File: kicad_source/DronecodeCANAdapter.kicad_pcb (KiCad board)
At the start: 2 copper layers, 65 x 30 mm, 31 parts, among them CN1 RASPI-IO, CN2 691322310004, CN3 GH_SM04B-GHS-TB, CN4 GH_SM04B-GHS-TB, SW1 JS202011JCQN, U1 MCP2518FD, U2 TCAN332GDR, Y1 RH100-20.000-20-3030-TR

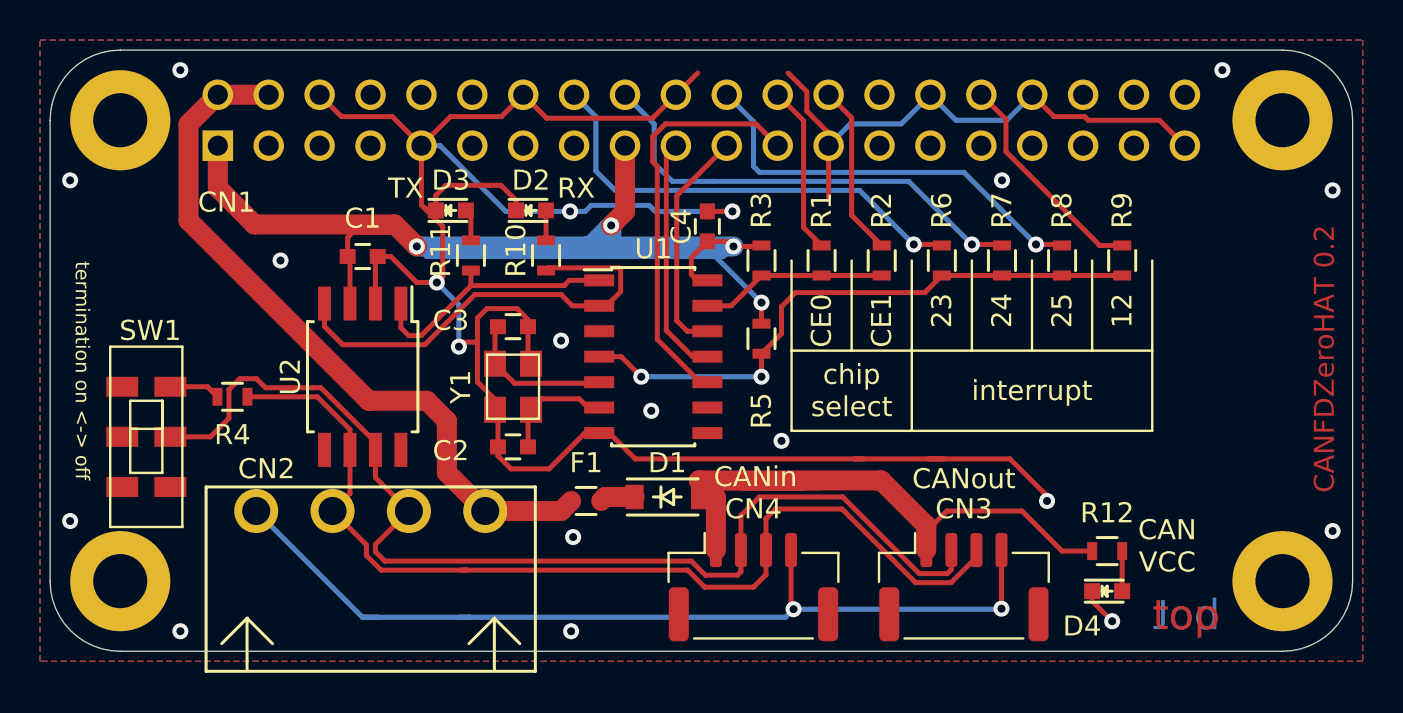
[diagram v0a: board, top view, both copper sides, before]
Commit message: updated schematic and layout
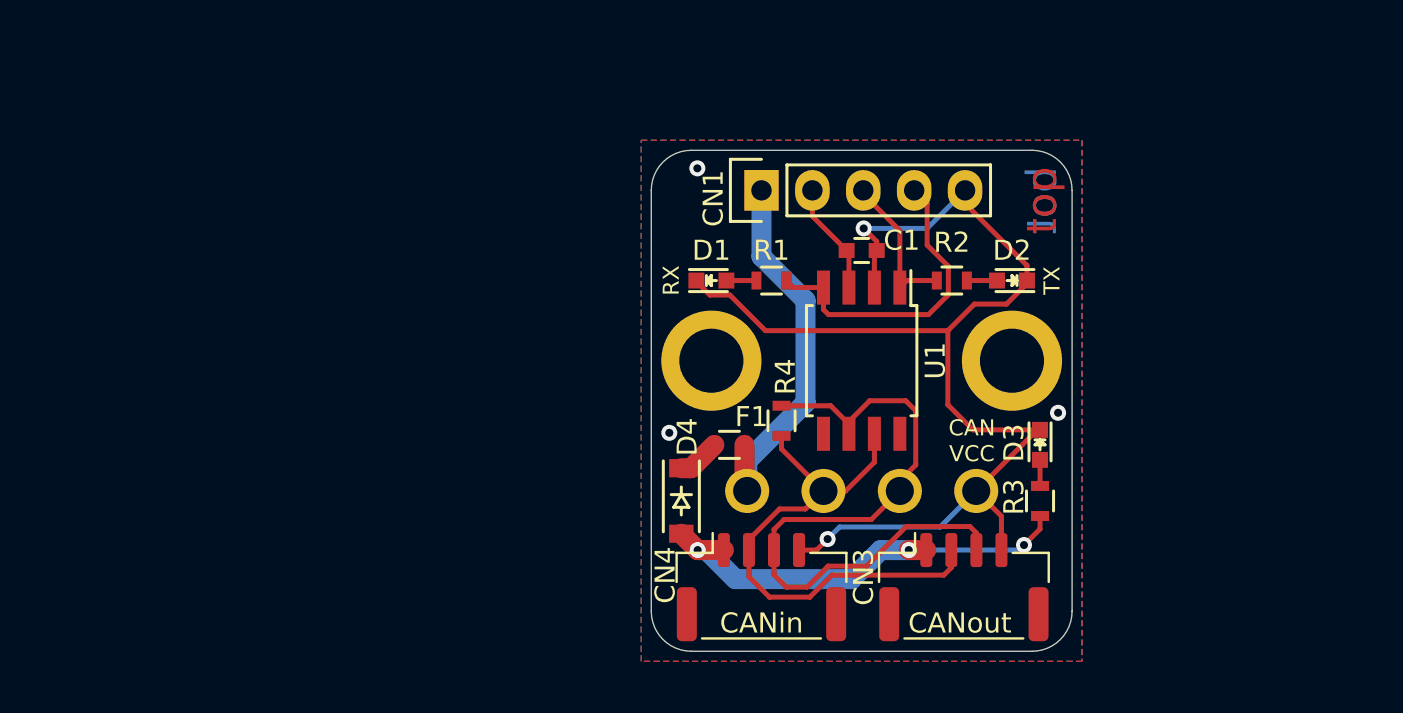
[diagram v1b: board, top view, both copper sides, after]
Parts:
- removed C2, C3: 22pF, capacitors:C_0603
- removed C4: 100nF, capacitors:C_0603
- removed the D3 at (127.5, 94.5)
- removed L2: Label, labels:generationmake_logo
- removed R10, R11: 1k, resistors:R_0603
- removed R12: 2k, resistors:R_0603
- removed R5: 10k, resistors:R_0603
- removed R6, R7, R9: DNI, resistors:R_0603
- removed R8: 0R, resistors:R_0603
- removed SW1: JS202011JCQN, mechanical-switches:CK_JS202011JCQN
- removed U2: TCAN332GDR, SOIC:SOIJ-8_5.3x5.3mm_Pitch1.27mm
- removed Y1: RH100-20.000-20-3030-TR, crystals:Crystal_SMD_3.2x2.5mm_4Pad
- added D1: 150060GS75000, LEDs:LED_0603, F.Cu at (140.5, 98.0)
- added MECH1: MHP_3.2_5.0, MECH_mounting_holes:MHP_3.2_5.0, F.Cu at (140.5, 102.0)
- added MECH2: MHP_3.2_5.0, MECH_mounting_holes:MHP_3.2_5.0, F.Cu at (155.5, 102.0)
- CN1: value RASPI-IO -> CONN_01X05; footprint MODULE_compute:RASPI_ZERO_HAT_EDGE -> pin_headers:Pin_Header_Straight_1x05
- CN2: moved to B.Cu
- D2: value 150060GS75000 -> 150060RS75000
- L1: footprint labels:generationmake_small_solder -> labels:generationmake_small_silk; moved to B.Cu
- R1: value 0R -> 1k
- R2: value DNI -> 1k
- R3: value 10k -> 2k
- R4: value 120R -> DNI
- U1: value MCP2518FD -> TCAN332GDR; footprint SOIC:SOIC-14_3.9x8.7mm_Pitch1.27mm -> SOIC:SOIJ-8_5.3x5.3mm_Pitch1.27mm
- moved R4 27.4 mm to (144.0, 105.0), turned to 270 degrees
- moved C1 24.9 mm to (148.0, 96.5)
- moved CN2 24.5 mm to (148.0, 108.5), turned to 180 degrees
- moved D2 24.3 mm to (155.5, 98.0), turned to 180 degrees
- moved L1 22.7 mm to (148.0, 100.8), turned to 180 degrees
- moved R3 18.4 mm to (156.9, 109.0), turned to 90 degrees
- moved U1 10.4 mm to (148.0, 102.0), turned to 270 degrees
- moved D3 8.03 mm to (156.9, 106.2), turned to 270 degrees
- moved F1 7.68 mm to (141.4, 106.2), turned to 180 degrees
- moved CN1 4.61 mm to (143.0, 93.5), turned to 90 degrees
- moved R2 3.64 mm to (152.5, 98.0), turned to 0 degrees
- moved R1 2.69 mm to (143.5, 98.0), turned to 180 degrees
- moved D4 0.73 mm to (139.0, 109.0), turned to 270 degrees
- moved CN4 0.40 mm to (143.0, 113.3)
- renumbered D4 to D3, D1 to D4
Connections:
- CN1 pad 1: +3V3 -> +5V
- CN1 pad 2: +5V -> +3V3
- CN1 pad 3: (no net) -> /CAN_TX
- CN1 pad 4: +5V -> /CAN_RX
- CN1 pad 5: (no net) -> GND
- D3 pad 2: Net-(D4-Pad2) -> Net-(D3-Pad2)
- R1 pad 1: /SPI_CE0 -> /CAN_RX
- R1 pad 2: /MCP2517_CS -> Net-(D1-Pad2)
- R2 pad 1: /MCP2517_CS -> /CAN_TX
- R2 pad 2: /SPI_CE1 -> Net-(D2-Pad2)
- R3 pad 1: +3V3 -> /CANVCC
- R3 pad 2: /MCP2517_CS -> Net-(D3-Pad2)
- R4 pad 2: Net-(R4-Pad2) -> /CANH
- U1 pad 2: /CAN_RX -> GND
- U1 pad 3: (no net) -> +3V3
- U1 pad 4: /MCP2517_INT -> /CAN_RX
- U1 pad 5: /OSC2 -> (no net)
- U1 pad 6: /OSC1 -> /CANL
- U1 pad 7: GND -> /CANH
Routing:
- net GND: track 185.6 -> 60.4 mm, vias 22 -> 5
- net +3V3: track 70.5 -> 5.61 mm, vias 4 -> 0
- net /MCP2517_INT: track 30.1 -> 0.00 mm, vias 2 -> 0
- net /CANH: track 55.6 -> 26.8 mm
- net /INTERRUPT_24: track 23.1 -> 0.00 mm, vias 1 -> 0
- net /INTERRUPT_23: track 23.1 -> 0.00 mm, vias 1 -> 0
- net /CANVCC: track 43.9 -> 22.7 mm, vias 0 -> 3
- net /INTERRUPT_25: track 21.2 -> 0.00 mm, vias 1 -> 0
- net /SPI_CLK: track 20.5 -> 0.00 mm
- net +5V: track 36.2 -> 19.5 mm
- net /CANL: track 50.2 -> 35.1 mm
- net /SPI_MOSI: track 12.0 -> 0.00 mm
- net /SPI_MISO: track 11.5 -> 0.00 mm
- net /INTERRUPT_12: track 11.1 -> 0.00 mm
- net /MCP2517_CS: track 9.33 -> 0.00 mm
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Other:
- board size 65 x 30 mm -> 21 x 25 mm
- board text added: "3V3"
- board text added: "5V"
- board text added: "CAN RX"
- board text added: "CAN TX"
- board text added: "Dronecode CANAdapter 0.1"
- board text removed: "12"
- board text removed: "23"
- board text removed: "24"
- board text removed: "25"
- board text removed: "CANFDZeroHAT 0.2"
- board text removed: "CE0"
- board text removed: "CE1"
- board text removed: "VCC"
- board text removed: "chip select"
- board text removed: "for Microchip MCP2517FD or MCP2518FD"
- board text removed: "interrupt"
- board text removed: "termination on <-> off"
